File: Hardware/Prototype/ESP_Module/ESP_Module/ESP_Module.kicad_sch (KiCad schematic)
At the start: 17 parts, among them J1 48037-0001, P1 USB_C_Plug, SW1 SW_SPST, SW2 SW_SPST, U1 AMS1117-3.3, U2 ESP32-S3-MINI-1-N8

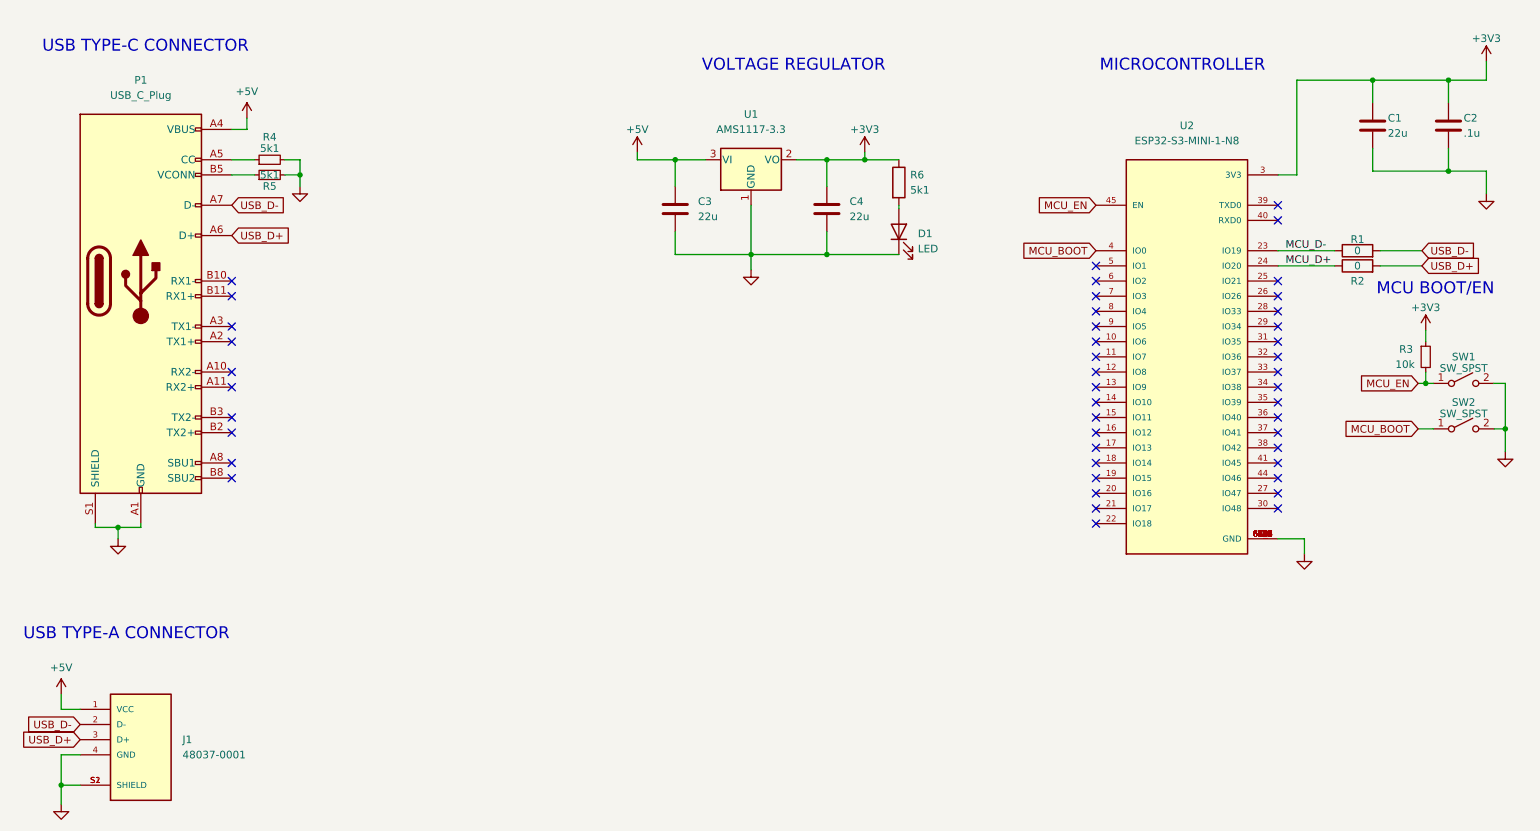
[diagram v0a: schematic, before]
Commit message: Finished prototyped module
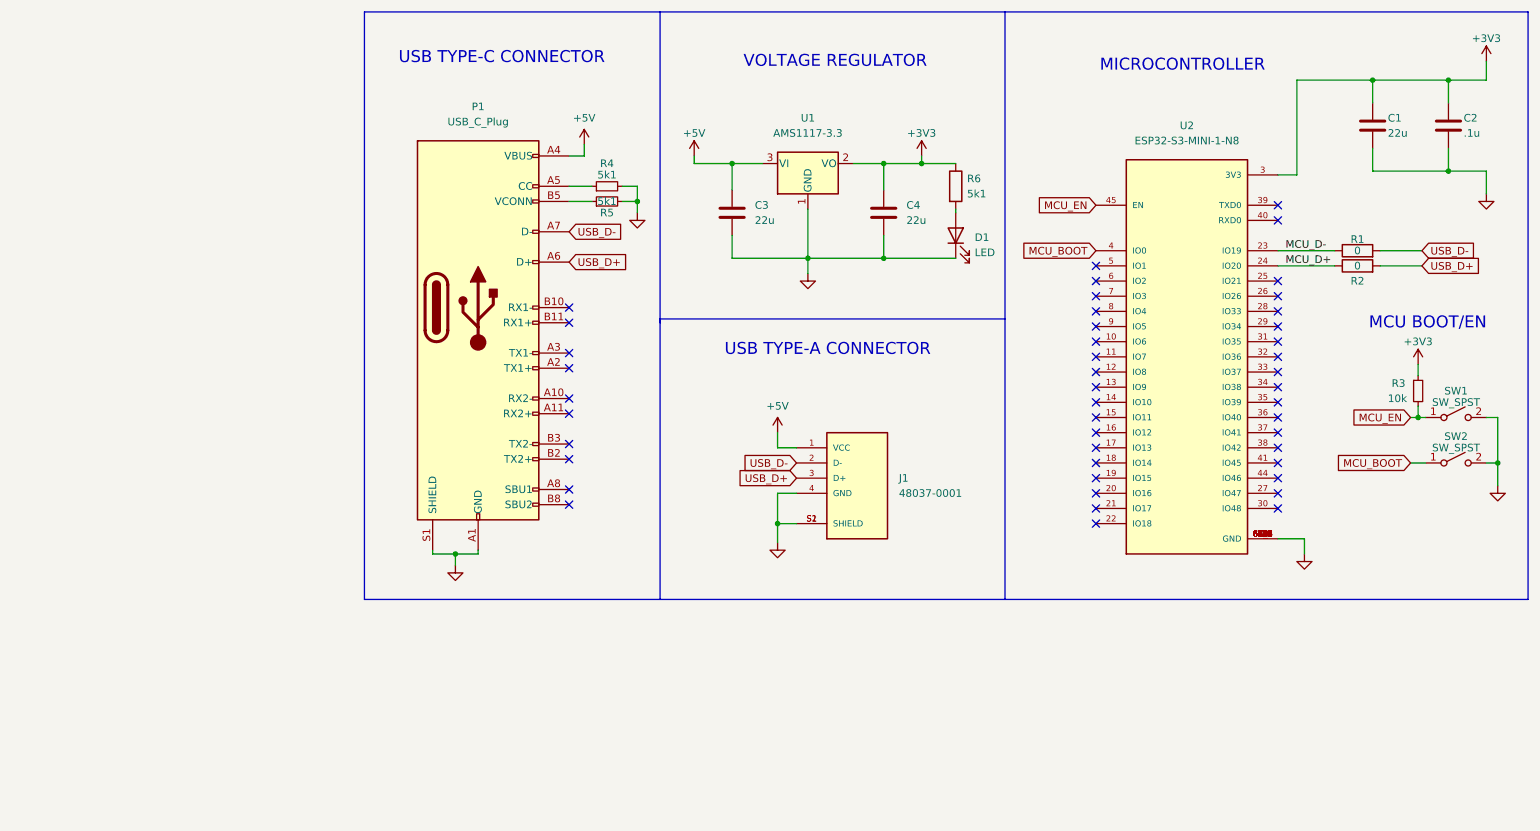
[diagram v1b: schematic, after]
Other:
- moved on the sheet: C3, C4, D1, J1, P1, R3, R4, R5, R6, SW1, SW2, U1
